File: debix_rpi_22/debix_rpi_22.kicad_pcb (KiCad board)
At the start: 2 copper layers, 71 x 12.5 mm, 2 parts, among them J1 Conn_01x24, J3 RPi 22 Pin MIPI CSI-2

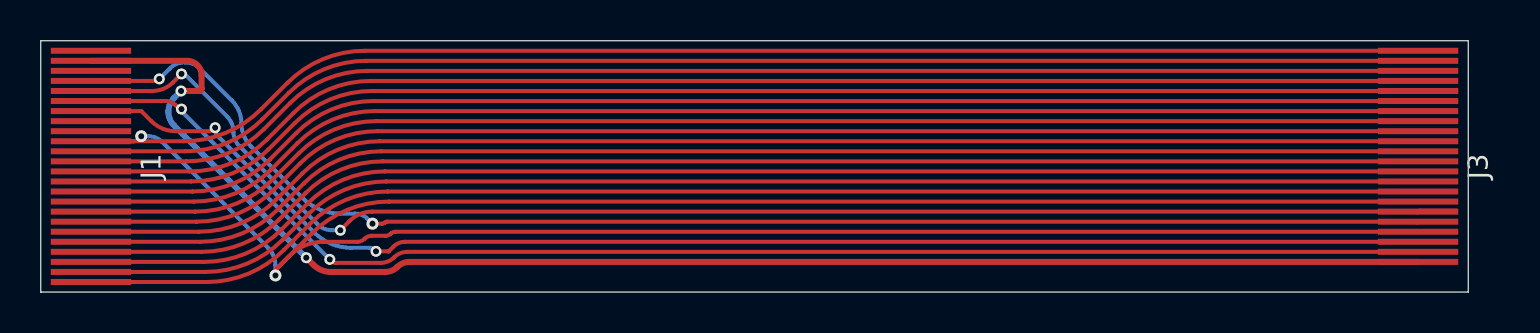
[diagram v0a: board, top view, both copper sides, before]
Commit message: ??
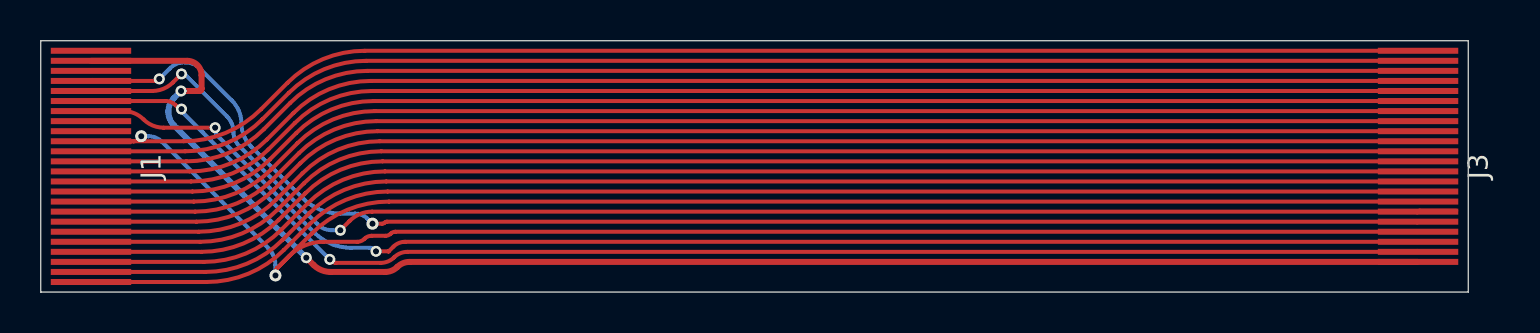
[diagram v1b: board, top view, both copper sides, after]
